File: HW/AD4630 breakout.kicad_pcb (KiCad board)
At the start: 2 copper layers, 30 x 30 mm, 4 parts, among them U1 AD4630-24BBCZ, U2 AMS1117-1.8, U3 TXS0108EPW, U4 TXS0108EPW

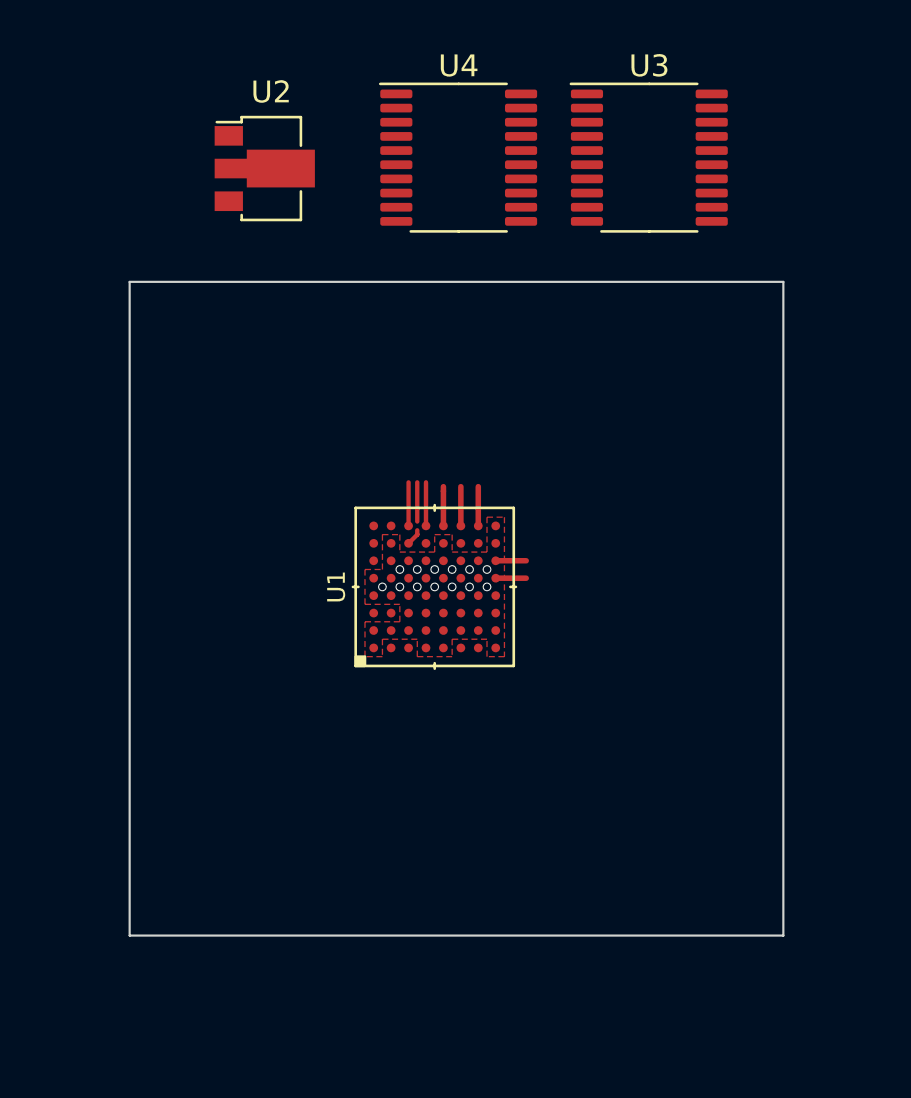
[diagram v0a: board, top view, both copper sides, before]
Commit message: PCB updated
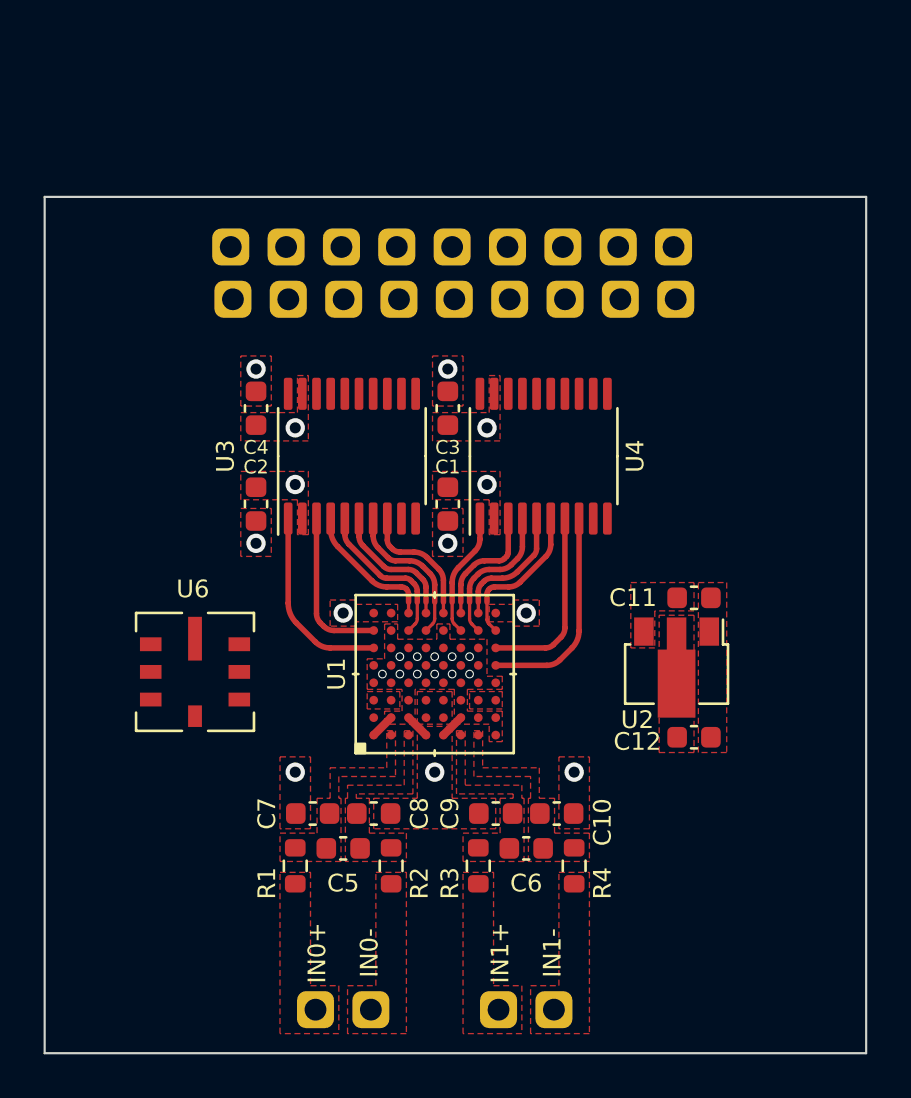
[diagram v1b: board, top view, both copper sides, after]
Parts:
- added C1: 10uF, Capacitor_SMD:C_0603_1608Metric, F.Cu at (144.6, 90.2)
- added C10: C, Capacitor_SMD:C_0603_1608Metric, F.Cu at (149.6, 104.4)
- added C11: 10uF, Capacitor_SMD:C_0603_1608Metric, F.Cu at (155.9, 94.5)
- added C12: 10uF, Capacitor_SMD:C_0603_1608Metric, F.Cu at (155.9, 100.9)
- added C2: 10uF, Capacitor_SMD:C_0603_1608Metric, F.Cu at (135.8, 90.2)
- added C3: 10uF, Capacitor_SMD:C_0603_1608Metric, F.Cu at (144.6, 85.8)
- added C4: 10uF, Capacitor_SMD:C_0603_1608Metric, F.Cu at (135.8, 85.8)
- added C5: C, Capacitor_SMD:C_0603_1608Metric, F.Cu at (139.8, 106.0)
- added C6: C, Capacitor_SMD:C_0603_1608Metric, F.Cu at (148.2, 106.0)
- added C7: C, Capacitor_SMD:C_0603_1608Metric, F.Cu at (138.4, 104.4)
- added C8: C, Capacitor_SMD:C_0603_1608Metric, F.Cu at (141.2, 104.4)
- added C9: C, Capacitor_SMD:C_0603_1608Metric, F.Cu at (146.8, 104.4)
- added J1: IN0, Connector_PinHeader_2.54mm:PinHeader_1x02_P2.54mm_Vertical, F.Cu at (138.5, 113.4)
- added J2: IN1, Connector_PinHeader_2.54mm:PinHeader_1x02_P2.54mm_Vertical, F.Cu at (146.9, 113.4)
- added J3: IO, Connector_PinHeader_2.54mm:PinHeader_1x09_P2.54mm_Vertical, F.Cu at (134.6, 78.4)
- added J4: IO, Connector_PinHeader_2.54mm:PinHeader_1x09_P2.54mm_Vertical, F.Cu at (134.7, 80.8)
- added R1: R, Resistor_SMD:R_0603_1608Metric, F.Cu at (137.6, 106.8)
- added R2: R, Resistor_SMD:R_0603_1608Metric, F.Cu at (142.0, 106.8)
- added R3: R, Resistor_SMD:R_0603_1608Metric, F.Cu at (146.0, 106.8)
- added R4: R, Resistor_SMD:R_0603_1608Metric, F.Cu at (150.4, 106.8)
- added U6: LTC6655BHLS8-5-PBF, LTC6655:LTC6655BHLS8-5-PBF, F.Cu at (133.0, 97.9)
- moved U2 29.7 mm to (155.1, 97.7), turned to -90 degrees
- moved U3 19.3 mm to (140.2, 88.0), turned to 90 degrees
- moved U4 14.2 mm to (149.0, 88.0), turned to 90 degrees
- moved U1 4.00 mm to (144.0, 98.0)
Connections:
- U1 pad A2: unconnected-(U1-PadA2) -> /REFIN
- U1 pad A6: unconnected-(U1-PadA6) -> /CNV
- U1 pad A7: unconnected-(U1-PadA7) -> /RST
- U1 pad B1: unconnected-(U1-PadB1) -> /IN0+
- U1 pad B8: +5V -> +1V8
- U1 pad C1: unconnected-(U1-PadC1) -> /IN0-
- U1 pad C7: unconnected-(U1-PadC7) -> /SDO3
- U1 pad C8: unconnected-(U1-PadC8) -> /SDO1
- U1 pad D2: unconnected-(U1-PadD2) -> /REF
- U1 pad D3: unconnected-(U1-PadD3) -> /REF
- U1 pad D7: unconnected-(U1-PadD7) -> /SDO2
- U1 pad D8: unconnected-(U1-PadD8) -> /SDO0
- U1 pad E2: unconnected-(U1-PadE2) -> /REF
- U1 pad E3: unconnected-(U1-PadE3) -> /REF
- U1 pad E8: unconnected-(U1-PadE8) -> /SCK OUT
- U1 pad F1: unconnected-(U1-PadF1) -> /IN1+
- U1 pad F7: unconnected-(U1-PadF7) -> /SDO6
- U1 pad F8: unconnected-(U1-PadF8) -> /SDO4
- U1 pad G1: unconnected-(U1-PadG1) -> /IN1-
- U1 pad G7: unconnected-(U1-PadG7) -> /SDO7
- U1 pad G8: unconnected-(U1-PadG8) -> /SDO5
- U1 pad H5: unconnected-(U1-PadH5) -> /CS
- U1 pad H6: unconnected-(U1-PadH6) -> /SDI
- U1 pad H7: unconnected-(U1-PadH7) -> /SCK
- U2 pad 1: unconnected-(U2-Pad1) -> GND
- U2 pad 2: unconnected-(U2-Pad2) -> +1V8
- U2 pad 3: unconnected-(U2-Pad3) -> +5V
- U3 pad 1: unconnected-(U3-Pad1) -> /CNV
- U3 pad 10: unconnected-(U3-Pad10) -> /OE
- U3 pad 11: unconnected-(U3-Pad11) -> GND
- U3 pad 12: unconnected-(U3-Pad12) -> Net-(U3-Pad12)
- U3 pad 13: unconnected-(U3-Pad13) -> Net-(U3-Pad13)
- U3 pad 14: unconnected-(U3-Pad14) -> Net-(U3-Pad14)
- U3 pad 15: unconnected-(U3-Pad15) -> Net-(U3-Pad15)
- U3 pad 16: unconnected-(U3-Pad16) -> Net-(U3-Pad16)
- U3 pad 17: unconnected-(U3-Pad17) -> Net-(U3-Pad17)
- U3 pad 18: unconnected-(U3-Pad18) -> Net-(U3-Pad18)
- U3 pad 19: unconnected-(U3-Pad19) -> +5V
- U3 pad 2: unconnected-(U3-Pad2) -> +1V8
- U3 pad 20: unconnected-(U3-Pad20) -> Net-(U3-Pad20)
- U3 pad 3: unconnected-(U3-Pad3) -> /RST
- U3 pad 4: unconnected-(U3-Pad4) -> /SDO1
- U3 pad 5: unconnected-(U3-Pad5) -> /SDO3
- U3 pad 6: unconnected-(U3-Pad6) -> /SDO0
- U3 pad 7: unconnected-(U3-Pad7) -> /SDO2
- U3 pad 8: unconnected-(U3-Pad8) -> /SCK OUT
- U4 pad 1: unconnected-(U4-Pad1) -> /SDO6
- U4 pad 10: unconnected-(U4-Pad10) -> /OE1
- U4 pad 11: unconnected-(U4-Pad11) -> GND
- U4 pad 12: unconnected-(U4-Pad12) -> Net-(U4-Pad12)
- U4 pad 13: unconnected-(U4-Pad13) -> Net-(U4-Pad13)
- U4 pad 14: unconnected-(U4-Pad14) -> Net-(U4-Pad14)
- U4 pad 15: unconnected-(U4-Pad15) -> Net-(U4-Pad15)
- U4 pad 16: unconnected-(U4-Pad16) -> Net-(U4-Pad16)
- U4 pad 17: unconnected-(U4-Pad17) -> Net-(U4-Pad17)
- U4 pad 18: unconnected-(U4-Pad18) -> Net-(U4-Pad18)
- U4 pad 19: unconnected-(U4-Pad19) -> +5V
- U4 pad 2: unconnected-(U4-Pad2) -> +1V8
- U4 pad 20: unconnected-(U4-Pad20) -> Net-(U4-Pad20)
- U4 pad 3: unconnected-(U4-Pad3) -> /SDO4
- U4 pad 4: unconnected-(U4-Pad4) -> /SDO7
- U4 pad 5: unconnected-(U4-Pad5) -> /SDO5
- U4 pad 6: unconnected-(U4-Pad6) -> /SCK
- U4 pad 7: unconnected-(U4-Pad7) -> /SDI
- U4 pad 8: unconnected-(U4-Pad8) -> /CS
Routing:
- net /CS: track 0.00 -> 9.81 mm
- net /CNV: track 0.00 -> 8.86 mm
- net /SDI: track 0.00 -> 8.66 mm
- net /RST: track 0.00 -> 7.39 mm
- net /SDO3: track 0.00 -> 7.26 mm
- net /SCK: track 0.00 -> 7.04 mm
- net /SDO2: track 0.00 -> 7.02 mm
- net /SDO7: track 0.00 -> 6.80 mm
- net /SDO1: track 0.00 -> 6.39 mm
- net /SDO0: track 0.00 -> 6.21 mm
- net /SCK OUT: track 0.00 -> 5.99 mm
- net /SDO5: track 0.00 -> 5.98 mm
- net /SDO4: track 0.00 -> 5.79 mm
- net /SDO6: track 0.00 -> 5.73 mm
- net GND: track 0.00 -> 3.39 mm, vias 13 -> 19
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- added copper zone on F.Cu, net +1V8
- added copper zone on F.Cu, net +5V
- added copper zone on F.Cu, net /IN0+
- added copper zone on F.Cu, net /IN0-
- added copper zone on F.Cu, net /IN1+
- added copper zone on F.Cu, net /IN1-
- added copper zone on F.Cu, net /REF
- added copper zone on F.Cu, net Net-(R1-Pad1)
- added copper zone on F.Cu, net Net-(R2-Pad1)
- added copper zone on F.Cu, net Net-(R3-Pad1)
- added copper zone on F.Cu, net Net-(R4-Pad1)
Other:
- board size 30 x 30 mm -> 37.7 x 39.3 mm
- board text added: "IN0+"
- board text added: "IN0-"
- board text added: "IN1+"
- board text added: "IN1-"
